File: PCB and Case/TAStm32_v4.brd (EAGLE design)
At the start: 50 x 100 mm, 55 parts, among them CN1 CA0612KRX7R7BB104, CN2 CA0612KRX7R7BB104, CN3 CA0612KRX7R7BB104, CN4 CA0612KRX7R7BB104, IC1 74HCT3G07DP-Q100H, IC2 74HCT3G07DP-Q100H, IC3 74AVCH4T245PW,118, IC4 74AVCH4T245PW,118, J1 ZX62D-B-5PA8, J10 RJSSE538002, J11 RJSSE538002, J12 SOICBITE, J13 CONSOLE_RESET, J2 UE27-AC54-100, J3 TSM-105-02-L-SHJ, J4 CONSOLE_RESET, J5 OLED128X64, J6 SAMTEC-TSM-116-01-X-SVJ, J7 SAMTEC-TSM-116-01-X-SVJ, U1 STM32F446RET6, U2 3.3V REG, Y1 8MHz

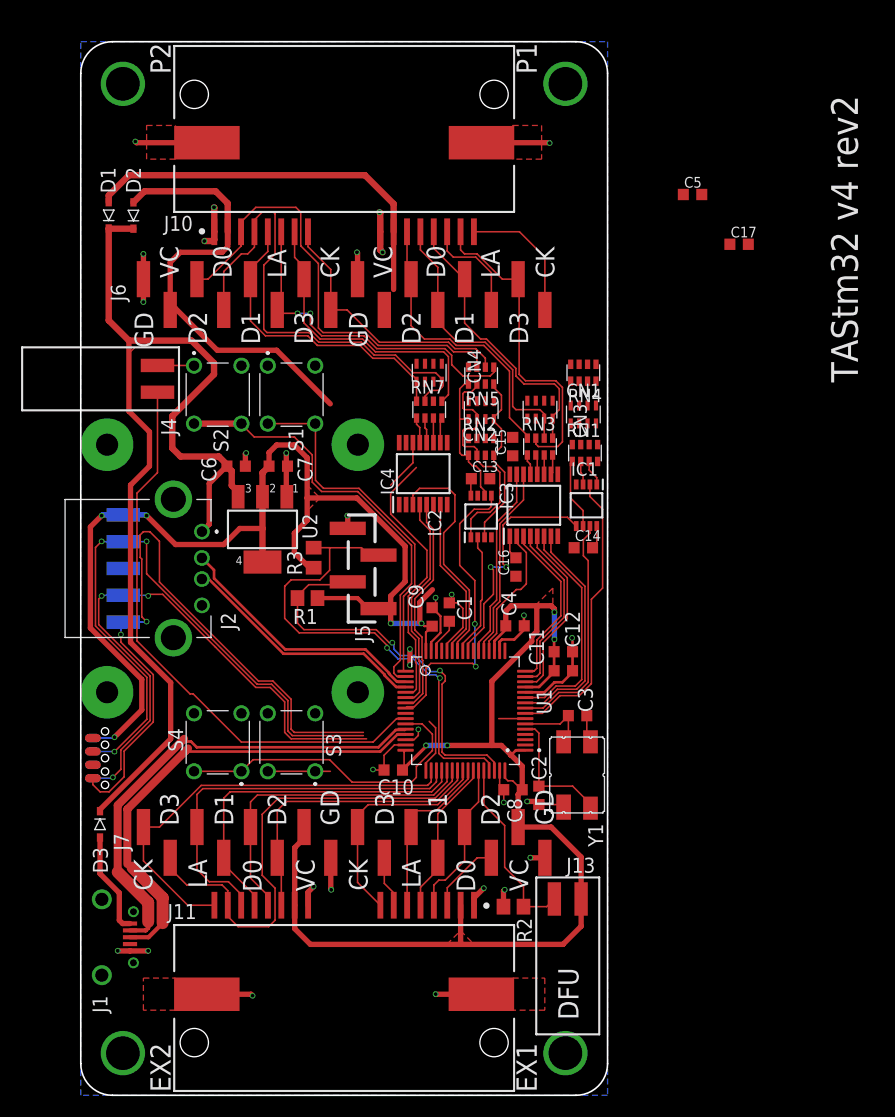
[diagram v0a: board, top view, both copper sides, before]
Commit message: no airwires!
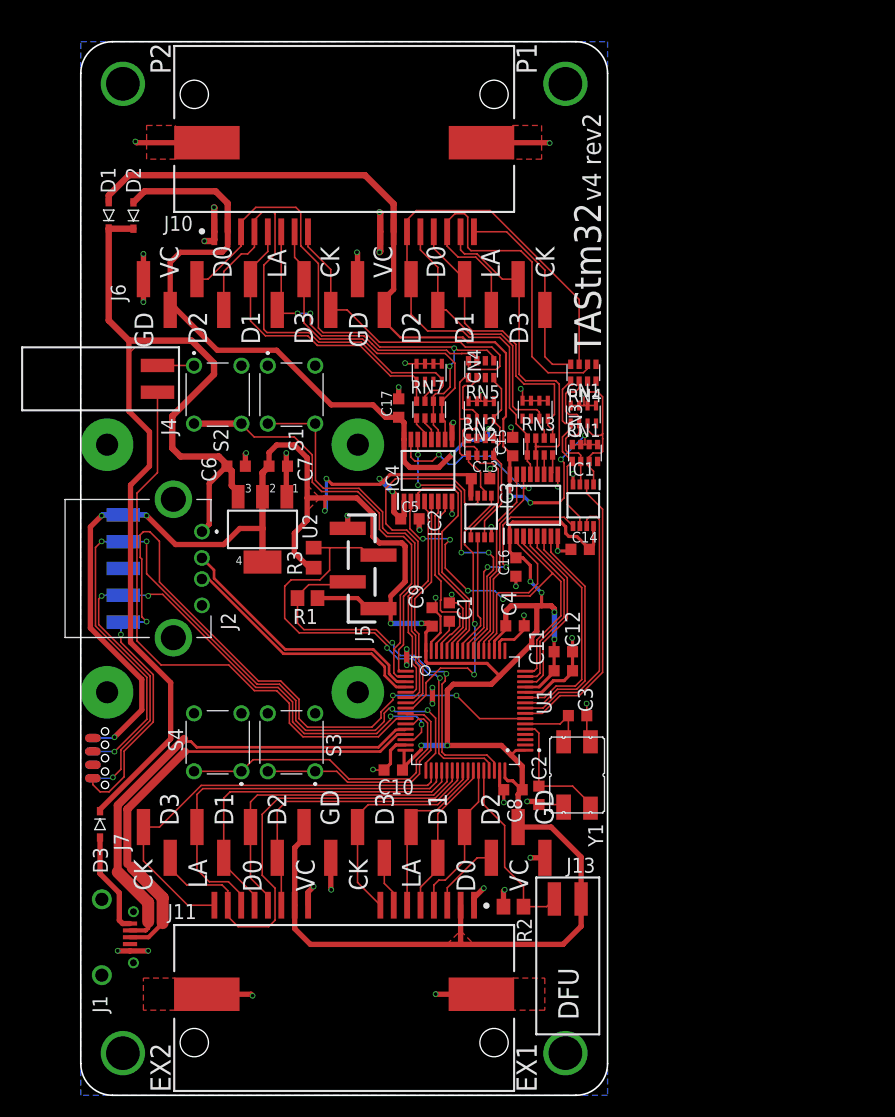
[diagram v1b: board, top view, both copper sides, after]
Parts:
- CN1, CN2, CN3, CN4: value CA0612KRX7R7BB104 -> 330pF
- RN1, RN2, RN5: value CTS742C083 -> 47K
- RN4, RN7: value CTS742C083 -> 47R
- moved C5 40.8 mm to (31.2, 54.7)
- moved C17 35.9 mm to (30.2, 65.2), turned to 90 degrees
- moved RN5 0.61 mm to (38.0, 68.9)
- moved IC4 0.55 mm to (33.0, 59.3)
- moved CN3 0.46 mm to (43.1, 65.1)
- moved C14 0.34 mm to (47.4, 51.8)
- moved IC1 0.30 mm to (47.7, 56.0)
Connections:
- removed net N$13: IC4.11, RN7.3
- removed net N$14: IC4.10, RN7.4
- removed net N$2: IC3.12, RN3.2
- removed net N$3: IC3.13, RN3.1
- net ENABLE_P2D2D3: now also U1.23
- net N$16: now also CN1.7, RN4.7; no longer CN1.8, RN4.8
- net N$17: now also CN1.5, RN4.5; no longer CN1.7, RN4.7
- net P1_CLOCK: now also RN4.4; no longer RN4.2
- net P1_D2: now also IC3.13, RN3.1
- net P1_D3: now also IC3.12, RN3.2
- net P1_LATCH: now also RN4.2; no longer RN4.1
- net P1_VCC: now also RN1.5, RN1.6, RN1.7, RN1.8
- net P2_CLOCK: now also RN5.4; no longer RN5.2
- net P2_D2: now also IC4.11, RN5.1, RN7.3; no longer RN5.3
- net P2_D2_3V_OUT: now also U1.29
- net P2_D3: now also IC4.10, RN7.4
- net P2_LATCH: now also RN5.3; no longer RN5.1
- net P2_VCC: now also RN2.5, RN2.6, RN2.7, RN2.8
- net V+: no longer RN1.6, RN1.7, RN1.8, RN2.5, RN2.6, RN2.7, RN2.8
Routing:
- net V+: track 227.7 -> 281.0 mm, vias 9 -> 15
- net P1_VCC: track 37.7 -> 84.0 mm, vias 0 -> 4
- net P1_D2: track 27.9 -> 59.1 mm
- net GND: track 103.1 -> 133.7 mm, vias 34 -> 52
- net P1_LATCH: track 11.4 -> 38.5 mm
- net P2_VCC: track 43.6 -> 68.6 mm, vias 0 -> 2
- net ENABLE_P2D2D3: track 4.90 -> 27.4 mm, vias 0 -> 4
- net DIR_D0D1: track 16.2 -> 38.4 mm, vias 0 -> 4
- net SWITCH3: track 5.94 -> 23.3 mm
- net P2_D2_3V_OUT: track 0.00 -> 17.0 mm
- net ENABLE_D0D1: track 18.3 -> 34.0 mm, vias 0 -> 2
- net NRST: track 68.0 -> 82.8 mm, vias 2 -> 4
- net N$16: track 2.48 -> 14.3 mm
- net N$18: track 2.28 -> 13.9 mm
- net P2_D2: track 43.0 -> 54.3 mm, vias 0 -> 2
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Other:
- board text added: "TAStm32"
- board text added: "v4 rev2"
- board text removed: "TAStm32 v4 rev2"
